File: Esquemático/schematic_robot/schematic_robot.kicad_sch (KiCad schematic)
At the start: 19 parts, among them J1 Conn_01x04_Pin, J2 Conn_01x01_Socket, J3 Conn_01x01_Socket, J4 Conn_01x01_Socket, J5 Conn_01x01_Socket, J6 Conn_01x01_Socket, J7 Conn_01x01_Socket, J8 Conn_01x01_Socket, J9 Conn_01x01_Socket, M1 Motor_Servo, M2 Motor_Servo, M3 Motor_Servo, M4 Motor_Servo, M5 Motor_Servo, U1 TB6600, U2 ESP32-WROOM-32, U3 PCA9685PW

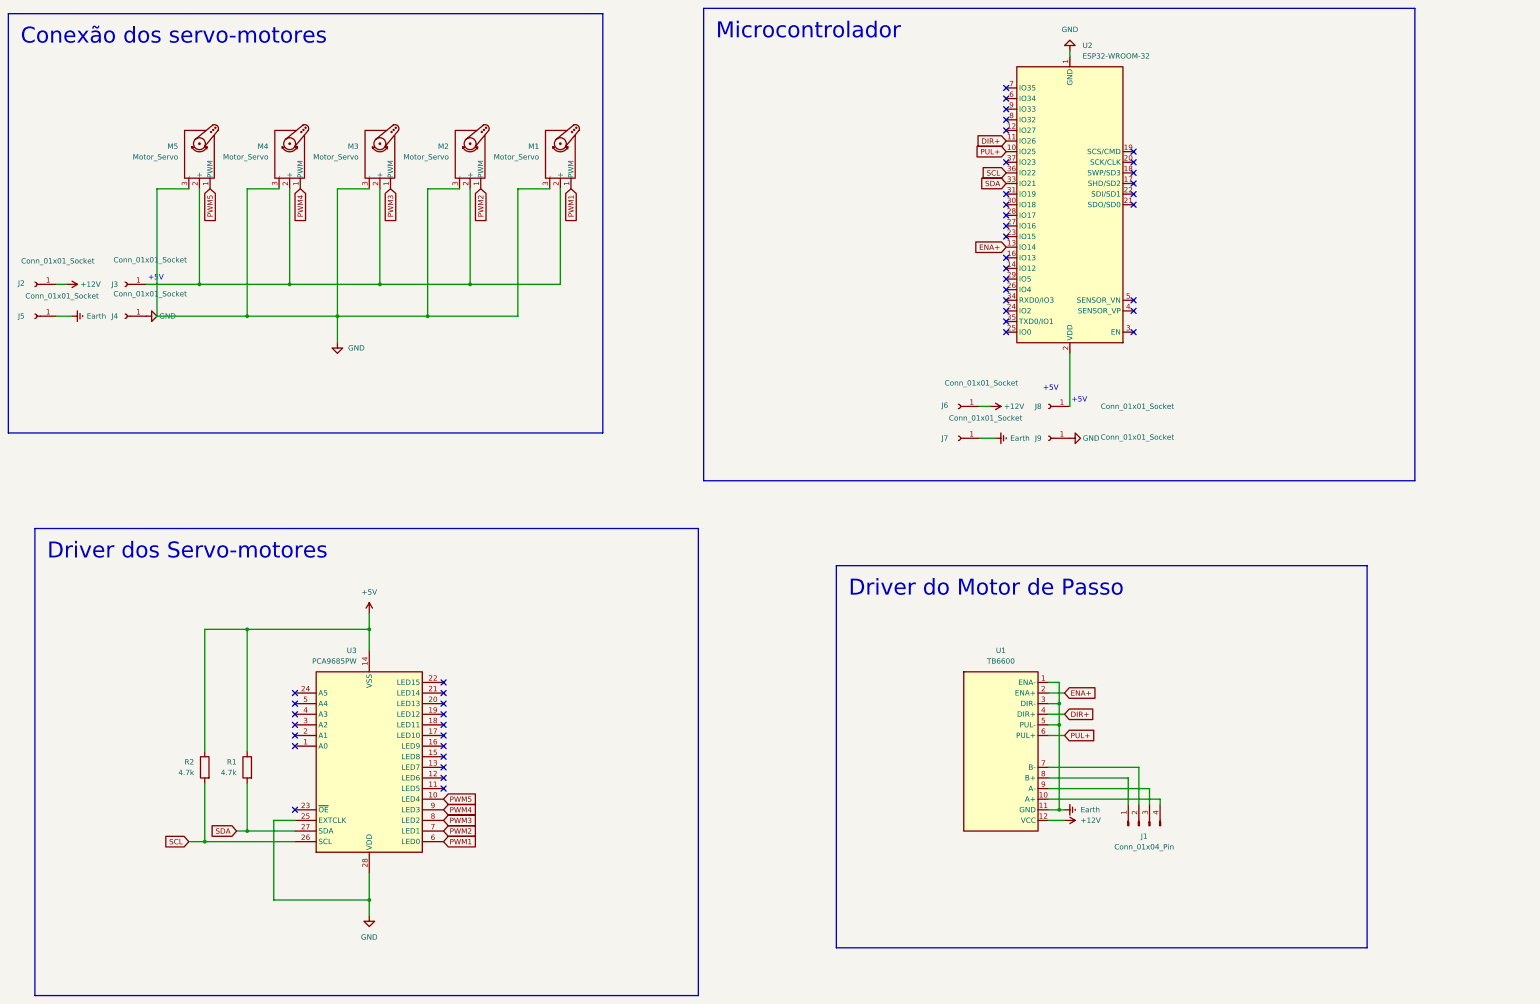
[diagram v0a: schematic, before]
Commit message: atualizei uns trem
esquema
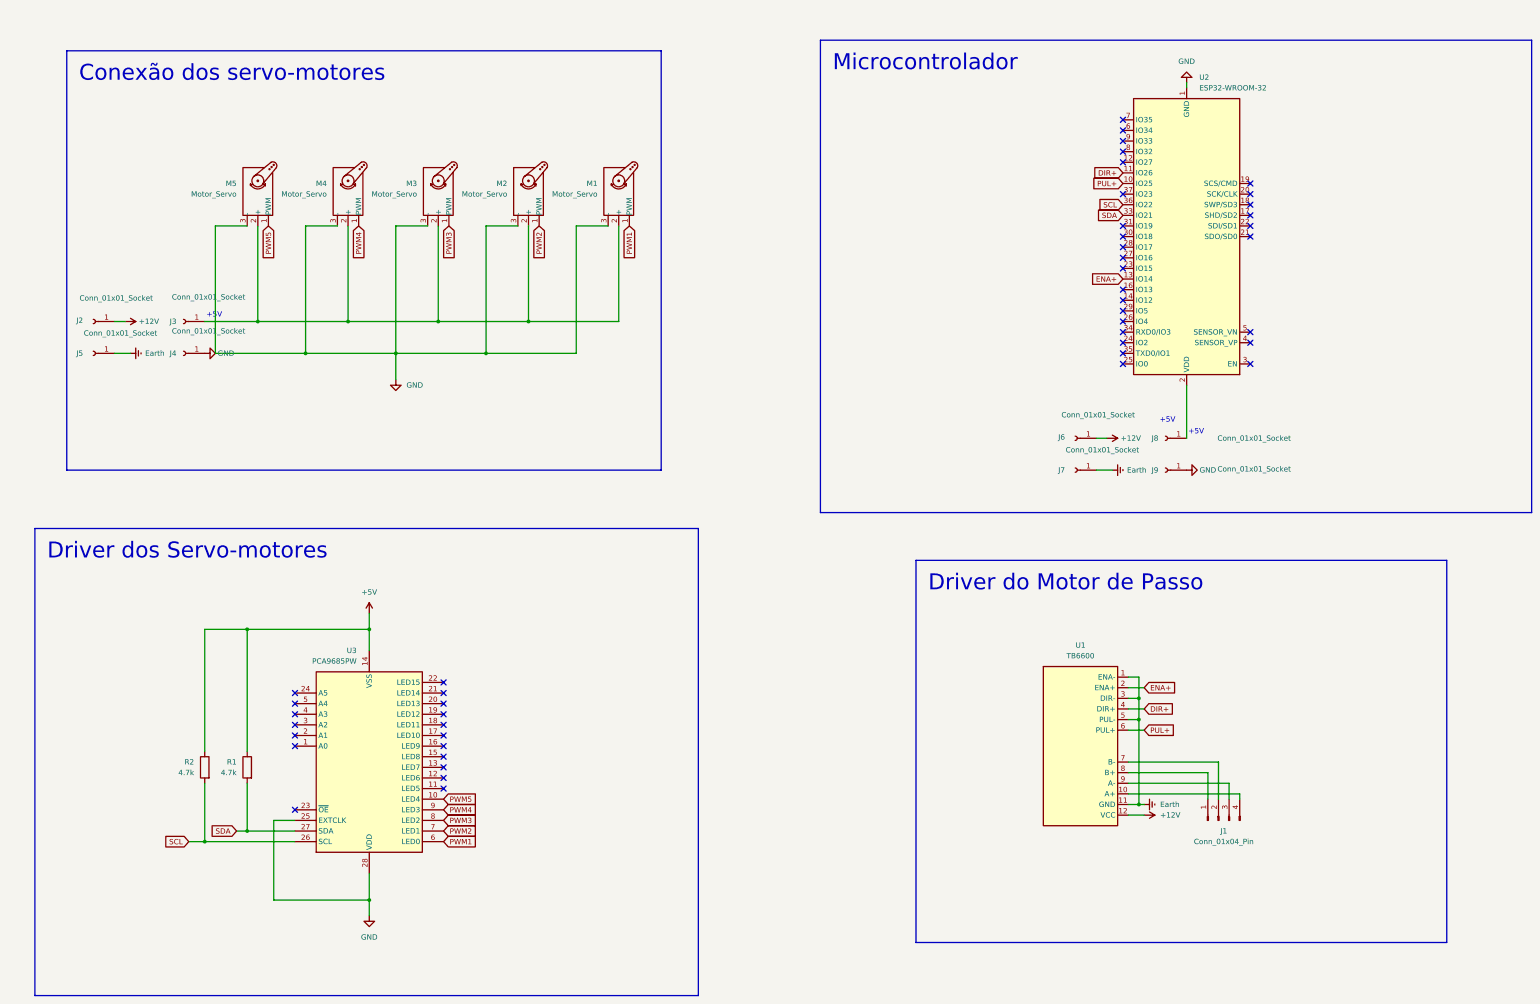
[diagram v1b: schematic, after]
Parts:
- J1: footprint (none) -> Connector_PinSocket_2.54mm:PinSocket_1x04_P2.54mm_Vertical
- J2, J3, J4, J5, J6, J7, J8, J9: footprint (none) -> Connector_PinSocket_2.54mm:PinSocket_1x01_P2.54mm_Vertical
- M1, M2, M3, M4, M5: footprint (none) -> Connector_JST:JST_EH_B3B-EH-A_1x03_P2.50mm_Vertical
- R1, R2: footprint (none) -> Resistor_THT:R_Axial_DIN0207_L6.3mm_D2.5mm_P10.16mm_Horizontal
- U1: footprint (none) -> Connector_PinSocket_2.54mm:PinSocket_1x12_P2.54mm_Vertical
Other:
- moved on the sheet: J1, J2, J3, J4, J5, J6, J7, J8, J9, M1, M2, M3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
